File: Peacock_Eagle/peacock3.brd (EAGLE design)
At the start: 100.2 x 80 mm, 110 parts, among them Q1 16M

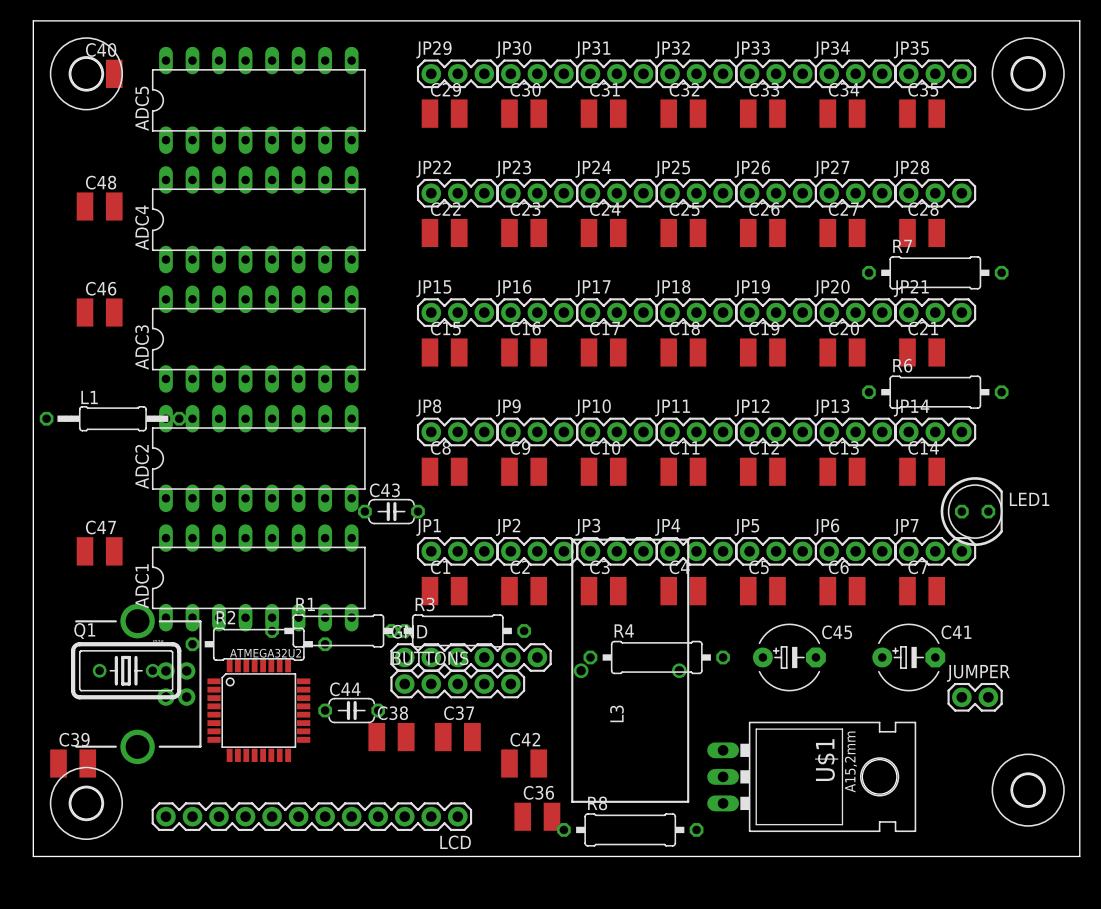
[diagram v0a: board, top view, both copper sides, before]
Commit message: routing done
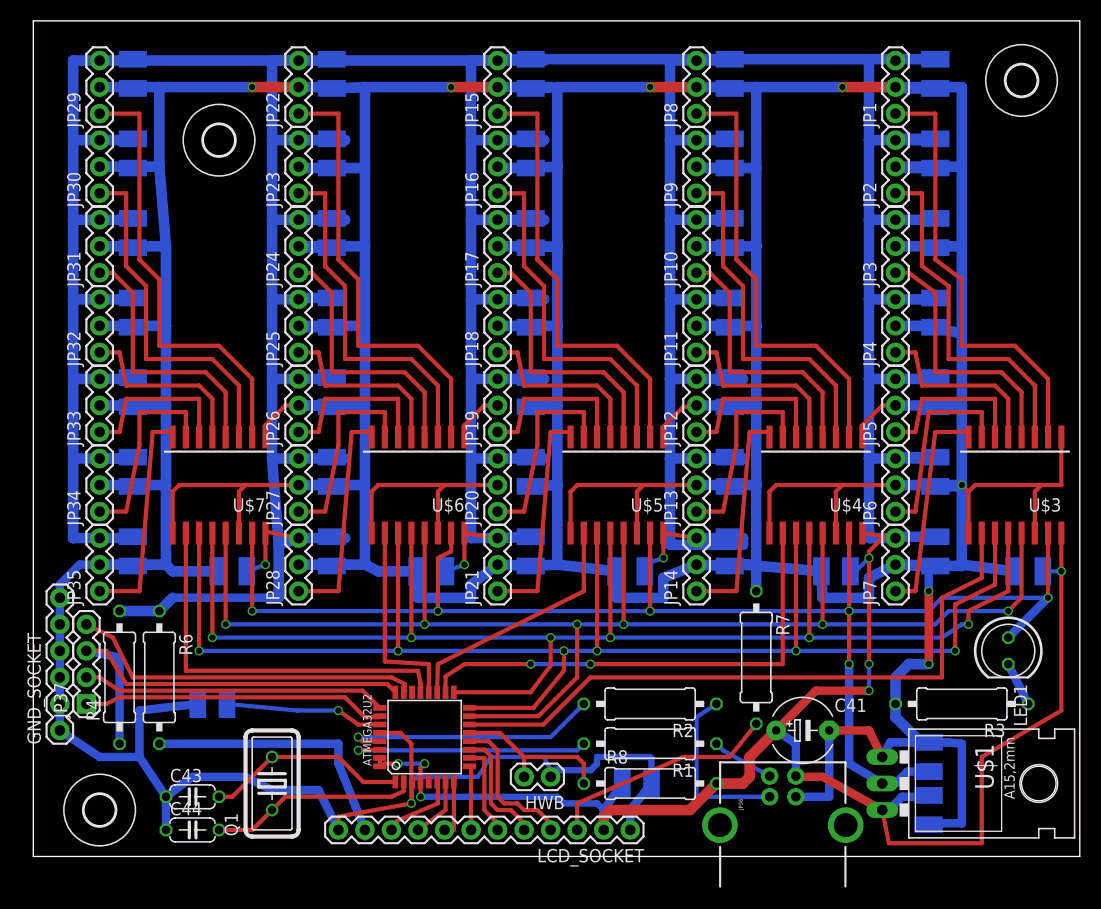
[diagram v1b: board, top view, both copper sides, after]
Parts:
- removed ADC1, ADC2, ADC3, ADC4, ADC5: MCP3208/DIP, mcp3208:DIL16
- removed BUTTONS: (no value), SparkFun-Connectors:1X05
- removed C45: 100uF, resistor:E5-6
- removed GND: (no value), SparkFun-Connectors:1X06
- removed H4: MOUNT-HOLE3.0, holes:3,0
- removed JUMPER: M02PTH, SparkFun-Connectors:1X02
- removed L1: 80R, resistor:0207/12
- removed L3: (no value), resistor:TJ5-U1
- removed LCD: M12PTH, SparkFun-Connectors:1X12
- added GND_SOCKET: (no value), SparkFun-Connectors:1X06
- added HWB: M02PTH, SparkFun-Connectors:1X02
- added JP37: (no value), SparkFun-Connectors:1X04
- added LCD_SOCKET: M12PTH, SparkFun-Connectors:1X12
- added U$3, U$4, U$5, U$6, U$7: MCP3208I/SL, myLibrary:SO-16DW
- C36, C37, C38, C39, C40: value 0.1uF -> 10uF
- U$1: device SparkFun-PowerIC:78XXL -> myLibrary:78XXL
- moved C40 100.9 mm to (95.2, 27.3), flipped to the bottom
- moved C48 95.3 mm to (85.7, 9.53), flipped to the bottom, turned to 90 degrees
- moved JP35 92.0 mm to (6.35, 25.4), turned to 90 degrees
- moved H3 89.5 mm to (94.6, 74.3)
- moved C35 86.4 mm to (9.53, 29.2), flipped to the bottom, turned to 270 degrees
- moved C47 83.1 mm to (85.7, 4.45), flipped to the bottom, turned to 270 degrees
- moved JP34 81.5 mm to (6.35, 33.0), turned to 90 degrees
- moved R6 79.2 mm to (12.1, 17.1), turned to 270 degrees
- moved H1 77.7 mm to (17.8, 68.6)
- moved C34 76.1 mm to (9.53, 36.8), flipped to the bottom, turned to 270 degrees
- moved C39 75.3 mm to (76.8, 27.3), flipped to the bottom
- moved JP33 71.1 mm to (6.35, 40.6), turned to 90 degrees
- moved JP28 69.7 mm to (25.4, 25.4), turned to 90 degrees
- moved C1 68.3 mm to (86.4, 74.9), flipped to the bottom, turned to 270 degrees
- moved C33 66.0 mm to (9.53, 44.5), flipped to the bottom, turned to 270 degrees
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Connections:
- removed net CS1: ADC1.10, ATMEGA32U2.14
- removed net CS2: ADC2.10, ATMEGA32U2.18
- removed net CS3: ADC3.10, ATMEGA32U2.19
- removed net CS4: ADC4.10, ATMEGA32U2.20
- removed net CS5: ADC5.10, ATMEGA32U2.21
- removed net N$10: JP36.VBUS, L1.2
- removed net N$21: ATMEGA32U2.26, BUTTONS.3
- removed net N$23: ATMEGA32U2.23, BUTTONS.1
- removed net N$31: ATMEGA32U2.22, LED1.A
- removed net N$49: C21.2, JP21.2
- removed net VCC: ATMEGA32U2.31, ATMEGA32U2.32, ATMEGA32U2.4, C41.+, C42.1, C45.+, L1.1, L3.2, LCD.2, R4.2, R6.1, R8.2
- removed net VDD: ADC1.16, ADC2.16, ADC3.16, ADC4.16, ADC5.16, C36.1, C37.1, C38.1, C39.1, C40.1
- new net N$39: ATMEGA32U2.14, U$3.10
- new net N$40: ATMEGA32U2.21, U$7.10
- new net N$44: ATMEGA32U2.20, U$6.10
- new net N$47: ATMEGA32U2.18, U$4.10
- new net N$48: ATMEGA32U2.19, U$5.10
- net +3V3: now also LED1.A, U$3.15, U$4.15, U$5.15, U$6.15, U$7.15; no longer ADC1.15, ADC2.15, ADC3.15, ADC4.15, ADC5.15
- net +5V: now also ATMEGA32U2.31, ATMEGA32U2.32, ATMEGA32U2.4, C36.1, C37.1, C38.1, C39.1, C40.1, C41.+, C42.1, JP36.VBUS, LCD_SOCKET.2, R4.2, R6.1, R8.2, U$3.16, U$4.16, U$5.16, U$6.16, U$7.16; no longer L3.1
- net BIT0: now also LCD_SOCKET.7; no longer LCD.7
- net BIT1: now also LCD_SOCKET.8; no longer LCD.8
- net BIT2: now also LCD_SOCKET.9; no longer LCD.9
- net BIT3: now also LCD_SOCKET.10; no longer LCD.10
- net CLK: now also U$3.13, U$4.13, U$5.13, U$6.13, U$7.13; no longer ADC1.13, ADC2.13, ADC3.13, ADC4.13, ADC5.13
- net ENABLE: now also LCD_SOCKET.6; no longer LCD.6
- net GND: now also ATMEGA32U2.28, C21.2, C43.1, C44.1, GND_SOCKET.1, GND_SOCKET.2, GND_SOCKET.3, GND_SOCKET.4, GND_SOCKET.5, GND_SOCKET.6, HWB.1, JP21.2, LCD_SOCKET.1, LCD_SOCKET.12, U$3.1, U$3.14, U$3.9, U$4.1, U$4.14, U$4.9, U$5.1, U$5.14, U$5.9, U$6.1, U$6.14, U$6.9, U$7.1, U$7.14, U$7.9; no longer ADC1.14, ADC1.8, ADC1.9, ADC2.14, ADC2.8, ADC2.9, ADC3.14, ADC3.8, ADC3.9, ADC4.14, ADC4.8, ADC4.9, ADC5.14, ADC5.8, ADC5.9, C45.-, GND.1, GND.2, GND.3, GND.4, GND.5, GND.6, JUMPER.1, LCD.1, LCD.12
- net HWB: now also HWB.2; no longer JUMPER.2
- net MISO: now also U$3.12, U$4.12, U$5.12, U$6.12, U$7.12; no longer ADC1.12, ADC2.12, ADC3.12, ADC4.12, ADC5.12
- net MOSI: now also U$3.11, U$4.11, U$5.11, U$6.11, U$7.11; no longer ADC1.11, ADC2.11, ADC3.11, ADC4.11, ADC5.11
- net N$1: now also ATMEGA32U2.26, JP37.1; no longer ATMEGA32U2.28, C43.1, C44.1
- net N$11: now also U$3.3; no longer ADC1.6
- net N$12: now also U$3.2; no longer ADC1.7
- net N$13: now also U$4.5; no longer ADC2.4
- net N$17: now also U$3.4; no longer ADC1.5
- net N$2: now also U$4.2; no longer ADC2.7
- net N$20: now also ATMEGA32U2.25, JP37.2; no longer ATMEGA32U2.5, BUTTONS.4
- net N$22: now also ATMEGA32U2.23, JP37.4; no longer ATMEGA32U2.25, BUTTONS.2
- net N$24: now also LCD_SOCKET.3; no longer LCD.3
- net N$25: now also U$4.4; no longer ADC2.5
- net N$26: now also JP37.3; no longer BUTTONS.5
- net N$27: now also LCD_SOCKET.11; no longer LCD.11
- net N$29: now also U$5.3; no longer ADC3.6
- net N$3: now also U$3.5; no longer ADC1.4
- net N$30: now also U$5.5; no longer ADC3.4
- net N$32: now also U$6.3; no longer ADC4.6
- net N$33: now also U$6.5; no longer ADC4.4
- net N$34: now also U$7.3; no longer ADC5.6
- net N$35: now also U$7.5; no longer ADC5.4
- net N$36: now also U$4.6; no longer ADC2.3
- net N$38: now also U$3.6; no longer ADC1.3
- net N$4: now also U$3.8; no longer ADC1.1
- net N$41: now also U$4.8; no longer ADC2.1
- net N$42: now also U$4.7; no longer ADC2.2
- net N$43: now also U$5.2; no longer ADC3.7
- net N$45: now also U$5.4; no longer ADC3.5
- net N$46: now also U$5.6; no longer ADC3.3
- net N$5: now also U$3.7; no longer ADC1.2
- net N$50: now also U$5.8; no longer ADC3.1
- net N$51: now also U$5.7; no longer ADC3.2
- net N$52: now also U$6.2; no longer ADC4.7
- net N$54: now also U$6.4; no longer ADC4.5
- net N$55: now also U$6.6; no longer ADC4.3
- net N$59: now also U$6.8; no longer ADC4.1
- net N$6: now also U$4.3; no longer ADC2.6
- net N$60: now also U$6.7; no longer ADC4.2
- net N$61: now also U$7.2; no longer ADC5.7
- net N$63: now also U$7.4; no longer ADC5.5
- net N$64: now also U$7.6; no longer ADC5.3
- net N$68: now also U$7.8; no longer ADC5.1
- net N$69: now also U$7.7; no longer ADC5.2
- net RS: now also LCD_SOCKET.4; no longer LCD.4
- net RW: now also LCD_SOCKET.5; no longer LCD.5
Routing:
- net GND: track 0.00 -> 905.2 mm, vias 0 -> 8
- net +5V: track 0.00 -> 768.2 mm, vias 0 -> 10
- net MOSI: track 0.00 -> 143.7 mm, vias 0 -> 6
- net +3V3: track 0.00 -> 142.3 mm, vias 0 -> 6
- net MISO: track 0.00 -> 137.1 mm, vias 0 -> 6
- net CLK: track 0.00 -> 135.3 mm, vias 0 -> 6
- net N$39: track 0.00 -> 63.3 mm
- net N$47: track 0.00 -> 46.7 mm, vias 0 -> 2
- net N$26: track 0.00 -> 43.2 mm
- net N$61: track 0.00 -> 42.6 mm
- net N$2: track 0.00 -> 42.6 mm
- net N$52: track 0.00 -> 42.6 mm
- net N$43: track 0.00 -> 42.6 mm
- net N$12: track 0.00 -> 42.4 mm
- net N$40: track 0.00 -> 37.5 mm
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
